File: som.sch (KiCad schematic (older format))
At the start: 39 parts, among them T2 BSS138APW, T4 BSS138APW, T5 BSS138APW

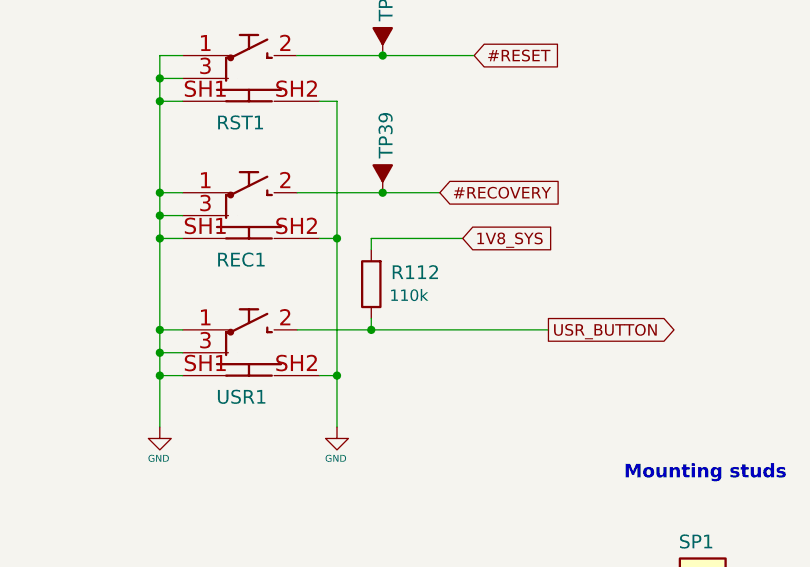
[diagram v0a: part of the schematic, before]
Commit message: Finish routing, cleanup silks
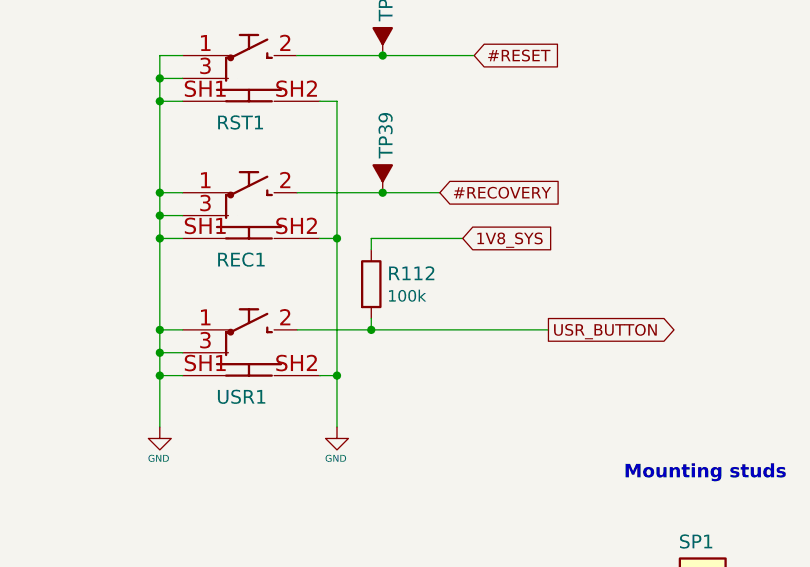
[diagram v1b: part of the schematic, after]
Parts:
- removed R112: R_110k_0603, jetson-nano-baseboard-footprints:0603-res, symbol jetson-nano-baseboard:R_110k_0603
- added R112: R_100k_0402, antmicro-footprints:0402-res, symbol antmicroResistors0402:R_100k_0402
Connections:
- net 1V8_SYS: now also R112.1
- net USR_BUTTON: now also R112.2
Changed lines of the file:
@@
 Wire Wire Line
 	11525 4075 11525 4025
-$Comp
-L jetson-nano-baseboard:R_110k_0603 R112
-U 1 1 62D721E3
-P 12450 7475
-F 0 "R112" V 12500 7175 60  0000 L CNN
-F 1 "R_110k_0603" H 12450 7325 60  0001 C CNN
-F 2 "jetson-nano-baseboard-footprints:0603-res" H 12650 7675 60  0001 L CNN
-F 3 "" H 12450 7475 50  0001 C CNN
-F 4 "TE" H 12650 7875 60  0001 L CNN "Manufacturer"
-F 5 "CPF0603B110KE1" H 12650 7775 60  0001 L CNN "MPN"
-F 6 "110k" V 12400 7225 50  0000 L CNN "Val"
-	1    12450 7475
-	0    -1   -1   0
-$EndComp
 Wire Wire Line
 	12125 7675 12450 7675
@@
 USR_BUTTON
 NoConn ~ 1875 10550
+$Comp
+L antmicroResistors0402:R_100k_0402 R112
+U 1 1 61ED8249
+P 12450 7475
+F 0 "R112" V 12405 7545 60  0000 L CNN
+F 1 "R_100k_0402" H 12450 7325 60  0001 C CNN
+F 2 "antmicro-footprints:0402-res" H 12650 7675 60  0001 L CNN
+F 3 "" H 12450 7475 50  0001 C CNN
+F 4 "VISHAY" H 12650 7875 60  0001 L CNN "Manufacturer"
+F 5 "CRCW0402100KFKEDHP" H 12650 7775 60  0001 L CNN "MPN"
+F 6 "100k" V 12503 7545 50  0000 L CNN "Val"
+	1    12450 7475
+	0    1    1    0
+$EndComp
 $EndSCHEMATC
